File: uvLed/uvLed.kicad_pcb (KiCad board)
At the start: 2 copper layers, 82 x 9 mm, 8 parts, among them J1 Conn_01x02

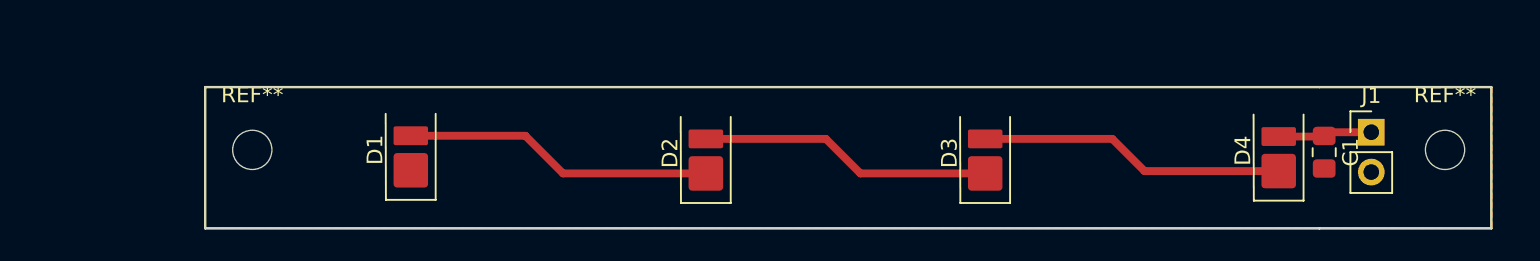
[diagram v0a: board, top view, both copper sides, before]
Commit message: update pcb
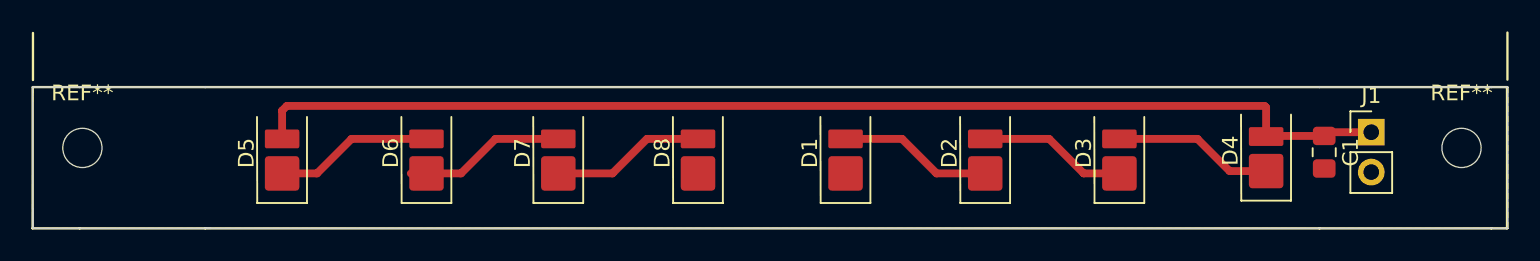
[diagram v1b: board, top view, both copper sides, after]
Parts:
- added D5: LED, uvLED:SMD-2, F.Cu at (112.5, 102.1)
- added D6: LED, uvLED:SMD-2, F.Cu at (121.7, 102.1)
- added D7: LED, uvLED:SMD-2, F.Cu at (130.1, 102.1)
- added D8: LED, uvLED:SMD-2, F.Cu at (138.9, 102.1)
- moved D1 27.7 mm to (148.3, 102.1)
- moved D2 17.8 mm to (157.2, 102.1)
- moved REF** 10.8 mm to (99.7, 101.8)
- moved D3 8.55 mm to (165.8, 102.1)
- moved REF** 1.06 mm to (187.6, 101.8)
- moved D4 0.80 mm to (175.2, 102.0)
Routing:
- net Net-(D4-A): track 6.01 -> 73.4 mm
- net Net-(D6-K): track 0.00 -> 10.3 mm
- net Net-(D7-K): track 0.00 -> 10.3 mm
- net Net-(D3-A): track 19.5 -> 9.40 mm
- net Net-(D1-A): track 19.8 -> 9.81 mm
- net Net-(D5-K): track 0.00 -> 9.11 mm
- net Net-(D2-A): track 18.7 -> 10.3 mm
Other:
- board size 82 x 9 mm -> 94 x 9 mm
